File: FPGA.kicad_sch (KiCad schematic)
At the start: 2 parts

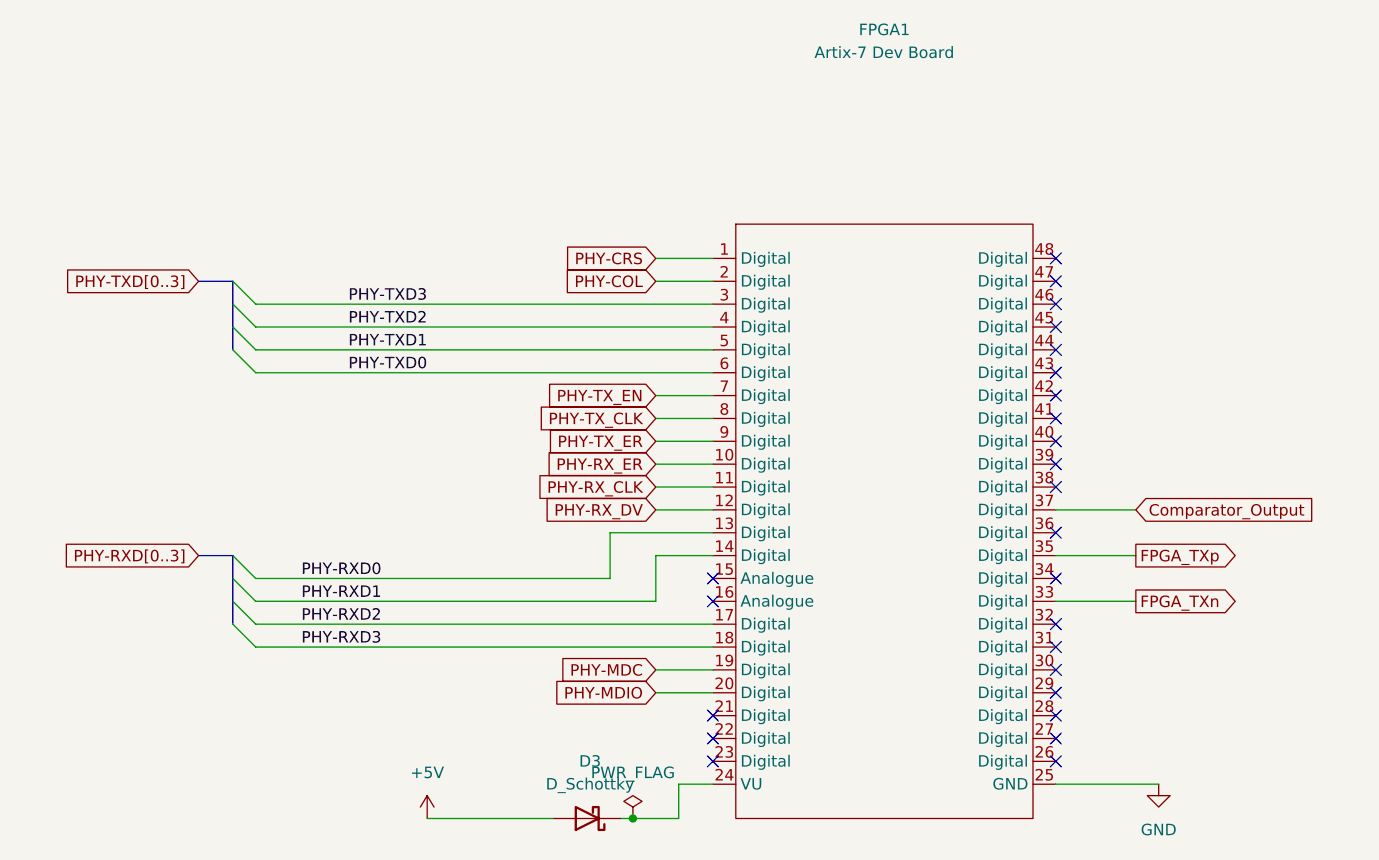
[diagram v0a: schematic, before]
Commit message: did lots of routing for phy
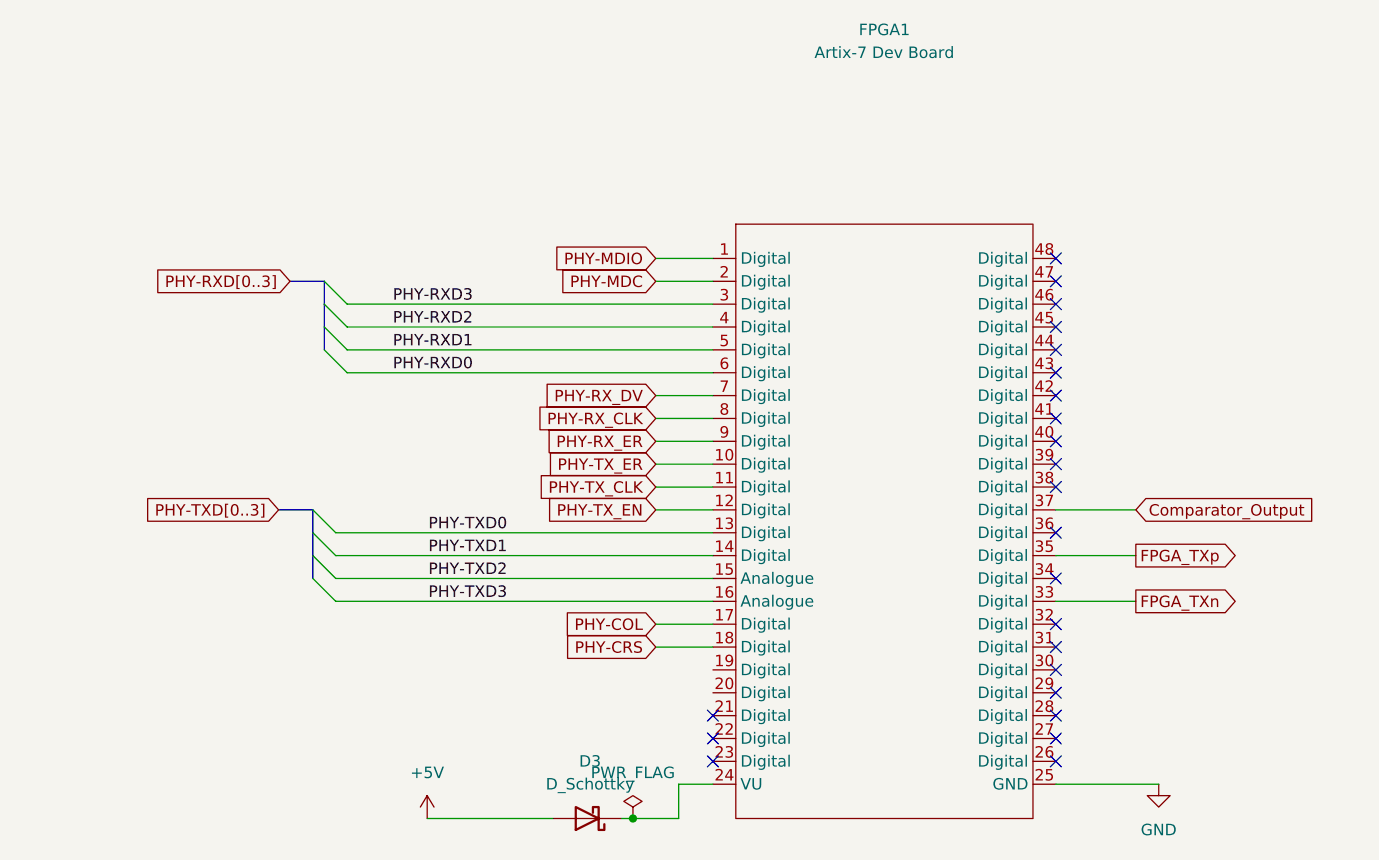
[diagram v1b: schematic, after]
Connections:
- net PHY-COL: now also FPGA1.17 (Digital); no longer FPGA1.2 (Digital)
- net PHY-CRS: now also FPGA1.18 (Digital); no longer FPGA1.1 (Digital)
- net PHY-MDC: now also FPGA1.2 (Digital); no longer FPGA1.19 (Digital)
- net PHY-MDIO: now also FPGA1.1 (Digital); no longer FPGA1.20 (Digital)
- net PHY-RXD0: now also FPGA1.6 (Digital); no longer FPGA1.13 (Digital)
- net PHY-RXD1: now also FPGA1.5 (Digital); no longer FPGA1.14 (Digital)
- net PHY-RXD2: now also FPGA1.4 (Digital); no longer FPGA1.17 (Digital)
- net PHY-RXD3: now also FPGA1.3 (Digital); no longer FPGA1.18 (Digital)
- net PHY-RX_CLK: now also FPGA1.8 (Digital); no longer FPGA1.11 (Digital)
- net PHY-RX_DV: now also FPGA1.7 (Digital); no longer FPGA1.12 (Digital)
- net PHY-RX_ER: now also FPGA1.9 (Digital); no longer FPGA1.10 (Digital)
- net PHY-TXD0: now also FPGA1.13 (Digital); no longer FPGA1.6 (Digital)
- net PHY-TXD1: now also FPGA1.14 (Digital); no longer FPGA1.5 (Digital)
- net PHY-TXD2: now also FPGA1.15 (Analogue); no longer FPGA1.4 (Digital)
- net PHY-TXD3: now also FPGA1.16 (Analogue); no longer FPGA1.3 (Digital)
- net PHY-TX_CLK: now also FPGA1.11 (Digital); no longer FPGA1.8 (Digital)
- net PHY-TX_EN: now also FPGA1.12 (Digital); no longer FPGA1.7 (Digital)
- net PHY-TX_ER: now also FPGA1.10 (Digital); no longer FPGA1.9 (Digital)
- no-connect marks 25 -> 23
